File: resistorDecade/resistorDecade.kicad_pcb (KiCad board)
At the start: 2 copper layers, 71 parts, among them J1 Screw_Terminal_01x02, J2 Conn_02x10_Odd_Even, J3 Conn_02x10_Odd_Even, J4 Conn_02x10_Odd_Even, J5 Conn_02x10_Odd_Even, J6 Conn_02x10_Odd_Even, J7 Conn_02x10_Odd_Even, J9 Conn_02x10_Odd_Even

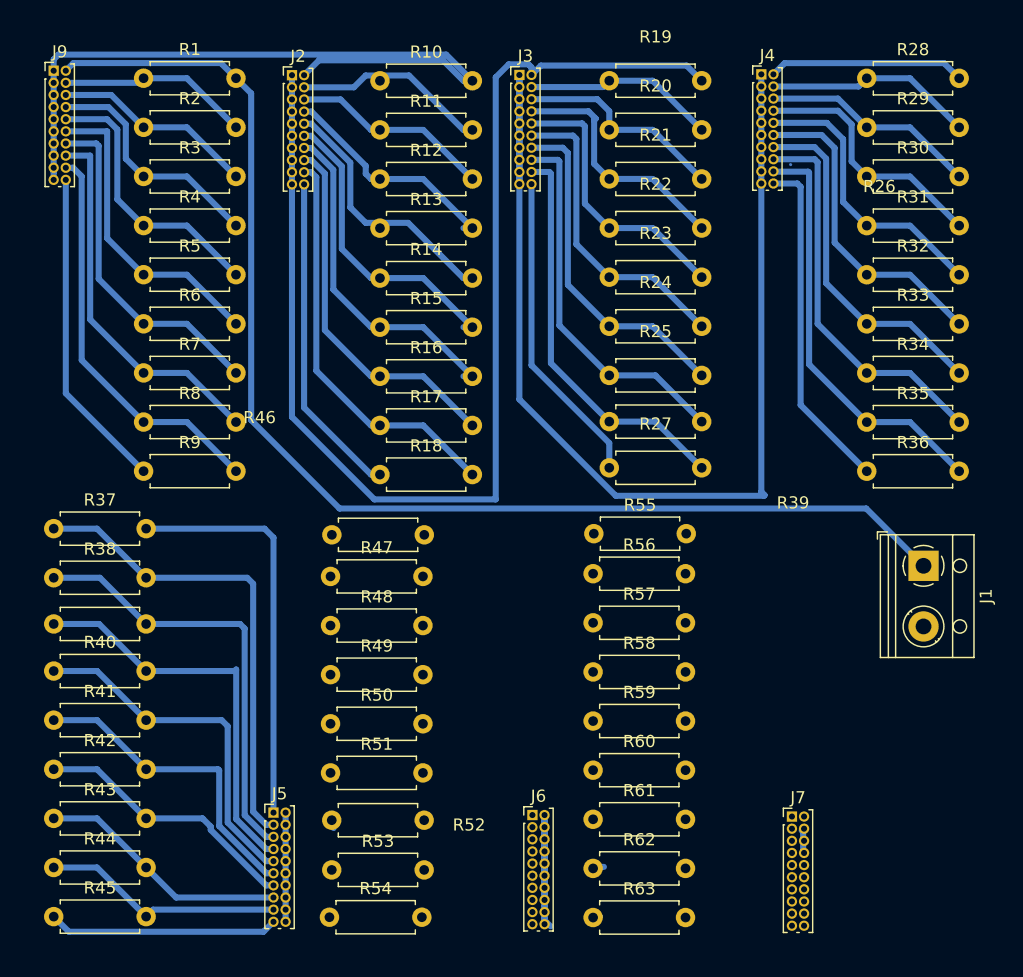
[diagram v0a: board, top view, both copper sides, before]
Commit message: Proyecto AD637 RMS
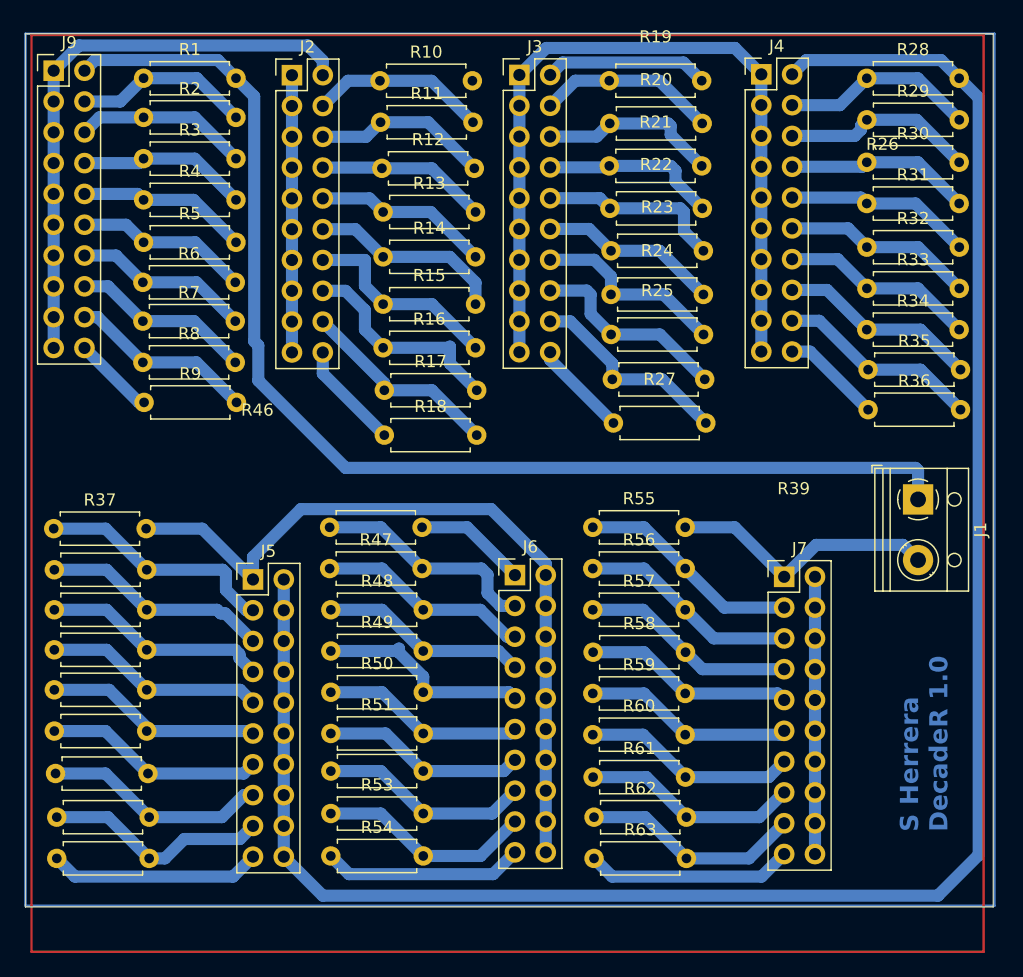
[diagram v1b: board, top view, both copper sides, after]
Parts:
- J2, J3, J4, J5, J6, J7, J9: footprint Connector_PinHeader_1.00mm:PinHeader_2x10_P1.00mm_Vertical -> Connector_PinHeader_2.54mm:PinHeader_2x10_P2.54mm_Vertical
- moved J6 19.8 mm to (134.9, 90.6)
- moved J7 19.8 mm to (157.1, 90.8)
- moved J5 19.3 mm to (113.3, 91.0)
- moved R9 5.67 mm to (104.3, 76.4)
- moved J1 5.49 mm to (168.1, 84.4)
- moved R36 5.08 mm to (164.0, 77.0)
- moved R54 5.05 mm to (119.7, 113.8)
- moved R8 4.92 mm to (104.2, 73.1)
- moved R63 4.88 mm to (141.4, 114.0)
- moved R45 4.81 mm to (97.1, 114.0)
- moved R53 4.65 mm to (119.7, 110.3)
- moved R35 4.33 mm to (164.0, 73.7)
- moved R7 4.27 mm to (104.2, 69.7)
- moved R62 4.23 mm to (141.4, 110.6)
- moved R44 4.16 mm to (97.1, 110.6)
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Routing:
- net Net-(J4-Pin_2): track 25.2 -> 162.5 mm
- net Net-(J2-Pin_1): track 101.6 -> 36.4 mm
- net Net-(J3-Pin_1): track 94.1 -> 67.5 mm
- net Net-(J1-Pin_2): track 0.00 -> 22.5 mm
- net Net-(J7-Pin_10): track 1.57 -> 22.9 mm
- net Net-(J9-Pin_20): track 26.7 -> 6.77 mm
- net Net-(J4-Pin_20): track 28.1 -> 8.25 mm
- net Net-(J5-Pin_3): track 39.2 -> 20.0 mm
- net Net-(J6-Pin_3): track 0.00 -> 18.9 mm
- net Net-(J7-Pin_3): track 0.00 -> 18.5 mm
- net Net-(J7-Pin_5): track 0.00 -> 18.2 mm
- net Net-(J3-Pin_20): track 26.1 -> 8.00 mm
- net Net-(J2-Pin_20): track 27.0 -> 8.92 mm
- net Net-(J7-Pin_15): track 0.00 -> 18.0 mm
- net Net-(J4-Pin_18): track 34.8 -> 16.9 mm
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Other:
- board outline added: 79.8 x 72 mm
- board text added: "S Herrera DecadeR 1.0"
